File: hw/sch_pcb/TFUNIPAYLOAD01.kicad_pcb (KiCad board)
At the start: 2 copper layers, 70.6 x 50.3 mm, 78 parts, among them J1 SM06B-GHS-TB, J2 SM08B-GHS-TB, J3 HEADER_2x03, J4 SM04B-GHS-TB, J5 HEADER_2x15, J6 SM07B-GHS-TB, M1 HOLE, M2 HOLE, M3 HOLE, M4 HOLE, Q1 BC817-25, Q2 BC817-25, SW1 SKRTLAE010, SW2 SKRTLAE010, U1 TPS631000DRLR, U2 ATMEGA1284P-AU, U3 TPS631000DRLR, Y1 8 MHz

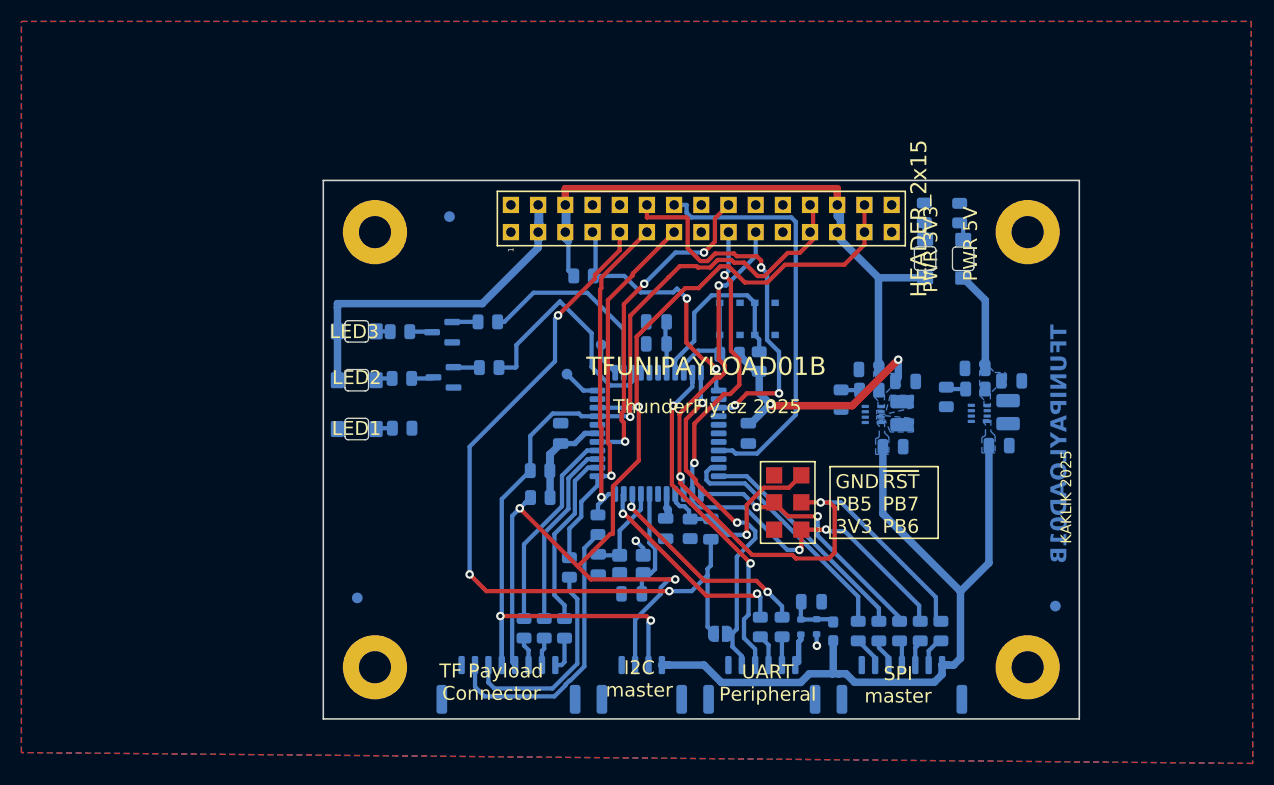
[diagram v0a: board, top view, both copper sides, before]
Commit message: Routed PCB.
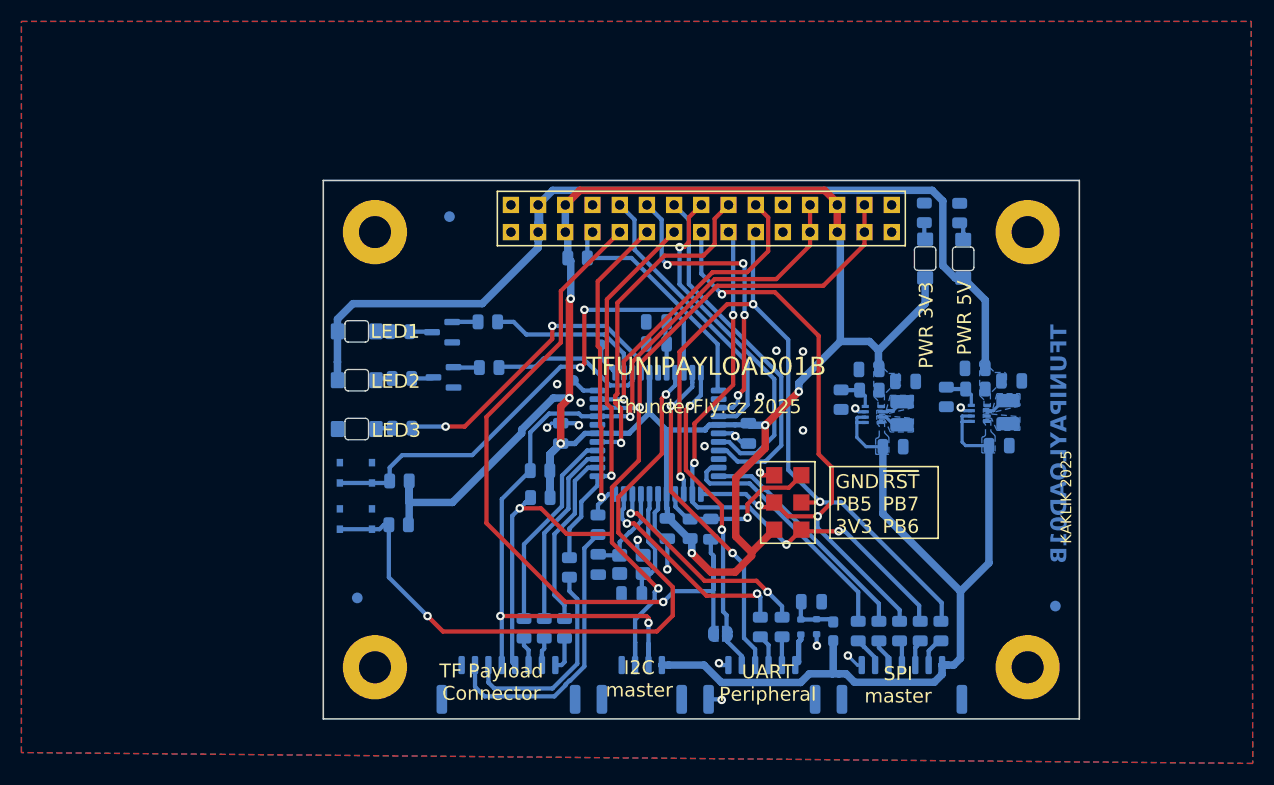
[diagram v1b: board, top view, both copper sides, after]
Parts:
- moved SW2 42.5 mm to (116.2, 111.5), turned to 0 degrees
- moved SW1 37.8 mm to (116.2, 107.2), turned to 0 degrees
- moved R3 37.0 mm to (120.2, 112.0), turned to 180 degrees
- moved R2 33.0 mm to (120.3, 107.9)
- moved R26 1.77 mm to (136.9, 87.1)
- moved TP1 0.84 mm to (136.6, 98.5)
- moved C10 0.15 mm to (145.3, 112.4)
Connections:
- net /PC5_D1 renamed /LED1
- net /PC6_D2 renamed /LED2
- net /PC7_D3 renamed /LED3
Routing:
- net +3.3V: track 97.3 -> 183.6 mm, vias 2 -> 6
- net /BTN_USER_B: track 17.3 -> 65.9 mm, vias 0 -> 2
- net +5V: track 44.9 -> 91.7 mm
- net /BTN_USER_A: track 9.05 -> 47.5 mm, vias 0 -> 2
- net /MOSI: track 24.8 -> 60.6 mm, vias 2 -> 3
- net /B0: track 0.00 -> 32.6 mm, vias 0 -> 1
- net /C0: track 0.00 -> 28.6 mm, vias 0 -> 1
- net /LED3: track 0.00 -> 27.9 mm, vias 0 -> 2
- net /A0: track 0.00 -> 26.7 mm
- net GND: track 2.73 -> 24.7 mm, vias 2 -> 19
- net +VSW: track 72.5 -> 84.6 mm
- net /LED2: track 22.3 -> 14.2 mm
- net /SDA: track 102.3 -> 94.2 mm
- net /A1: track 35.0 -> 28.8 mm, vias 3 -> 4
- net /SCL: track 89.7 -> 83.6 mm
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- added copper zone on B.Cu, net Net-(U3-LX1)
- added copper zone on B.Cu, net Net-(U3-LX2)
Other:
- rule pad_to_mask_clearance: 0.08 -> 0.05
